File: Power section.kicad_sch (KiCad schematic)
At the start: 14 parts, among them IC1 TPD4E001RDBVR, IC2 BQ24040DSQR, J1 USB4110-GF-A, J2 B03B-PASK-1(LF)(SN)

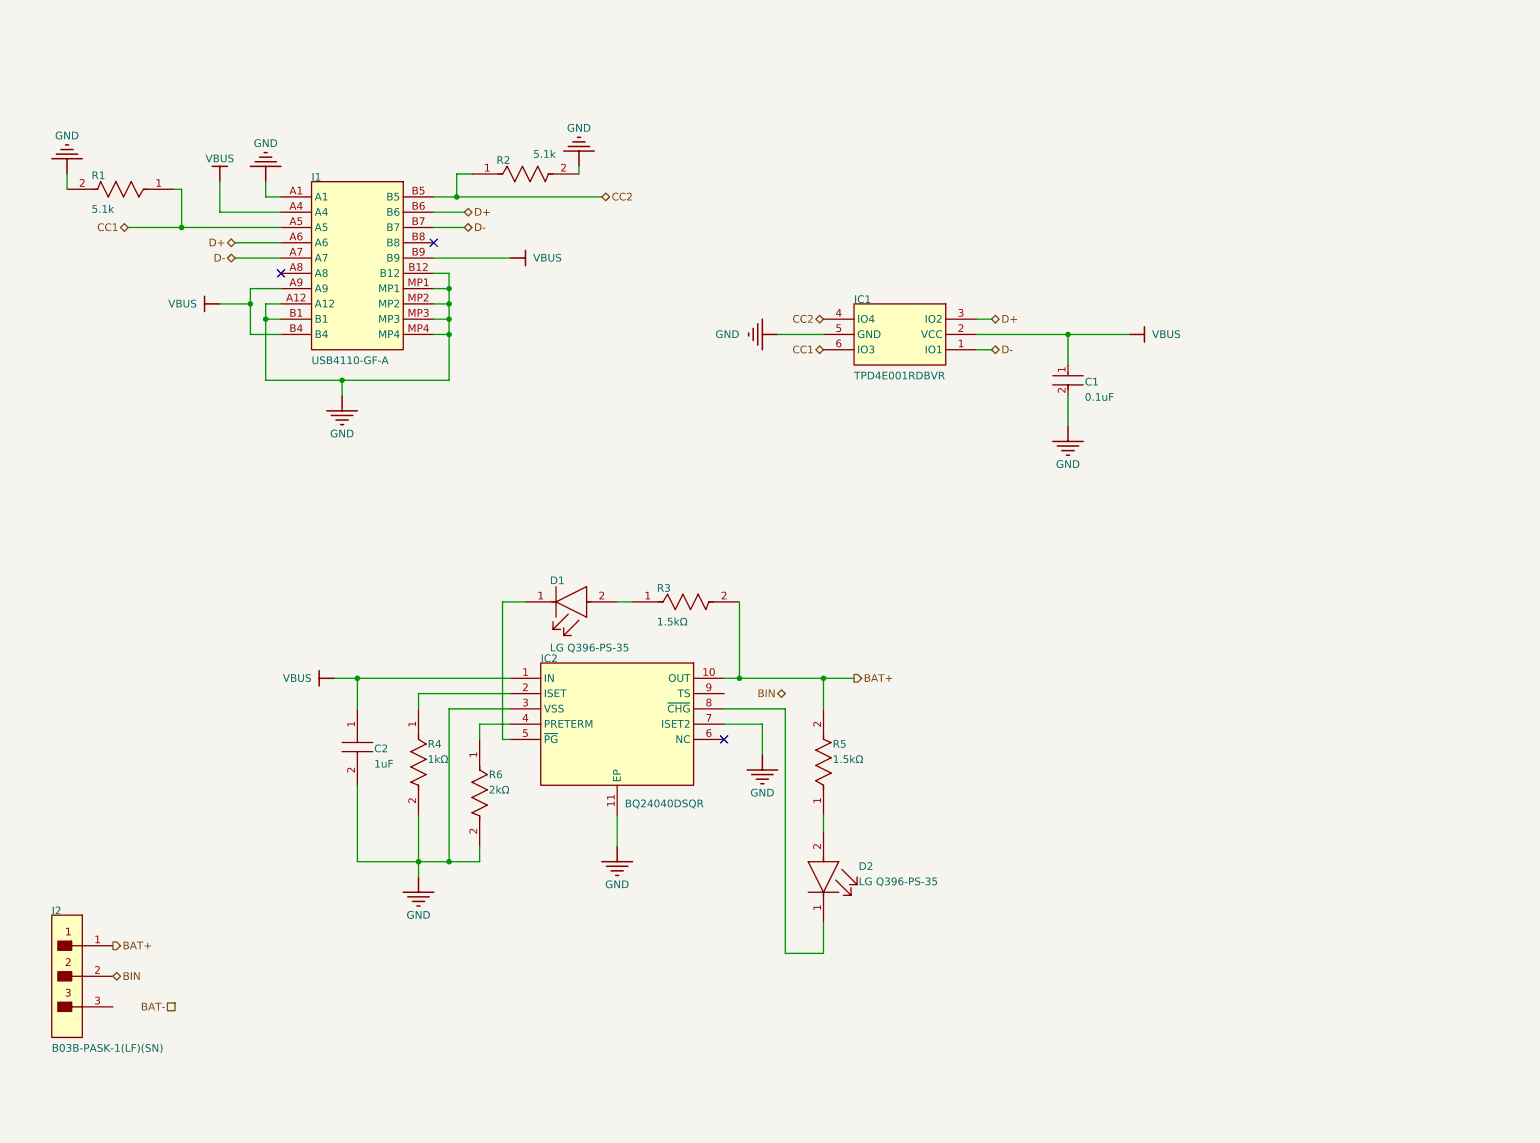
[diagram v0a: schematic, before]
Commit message: feat: schematic v1
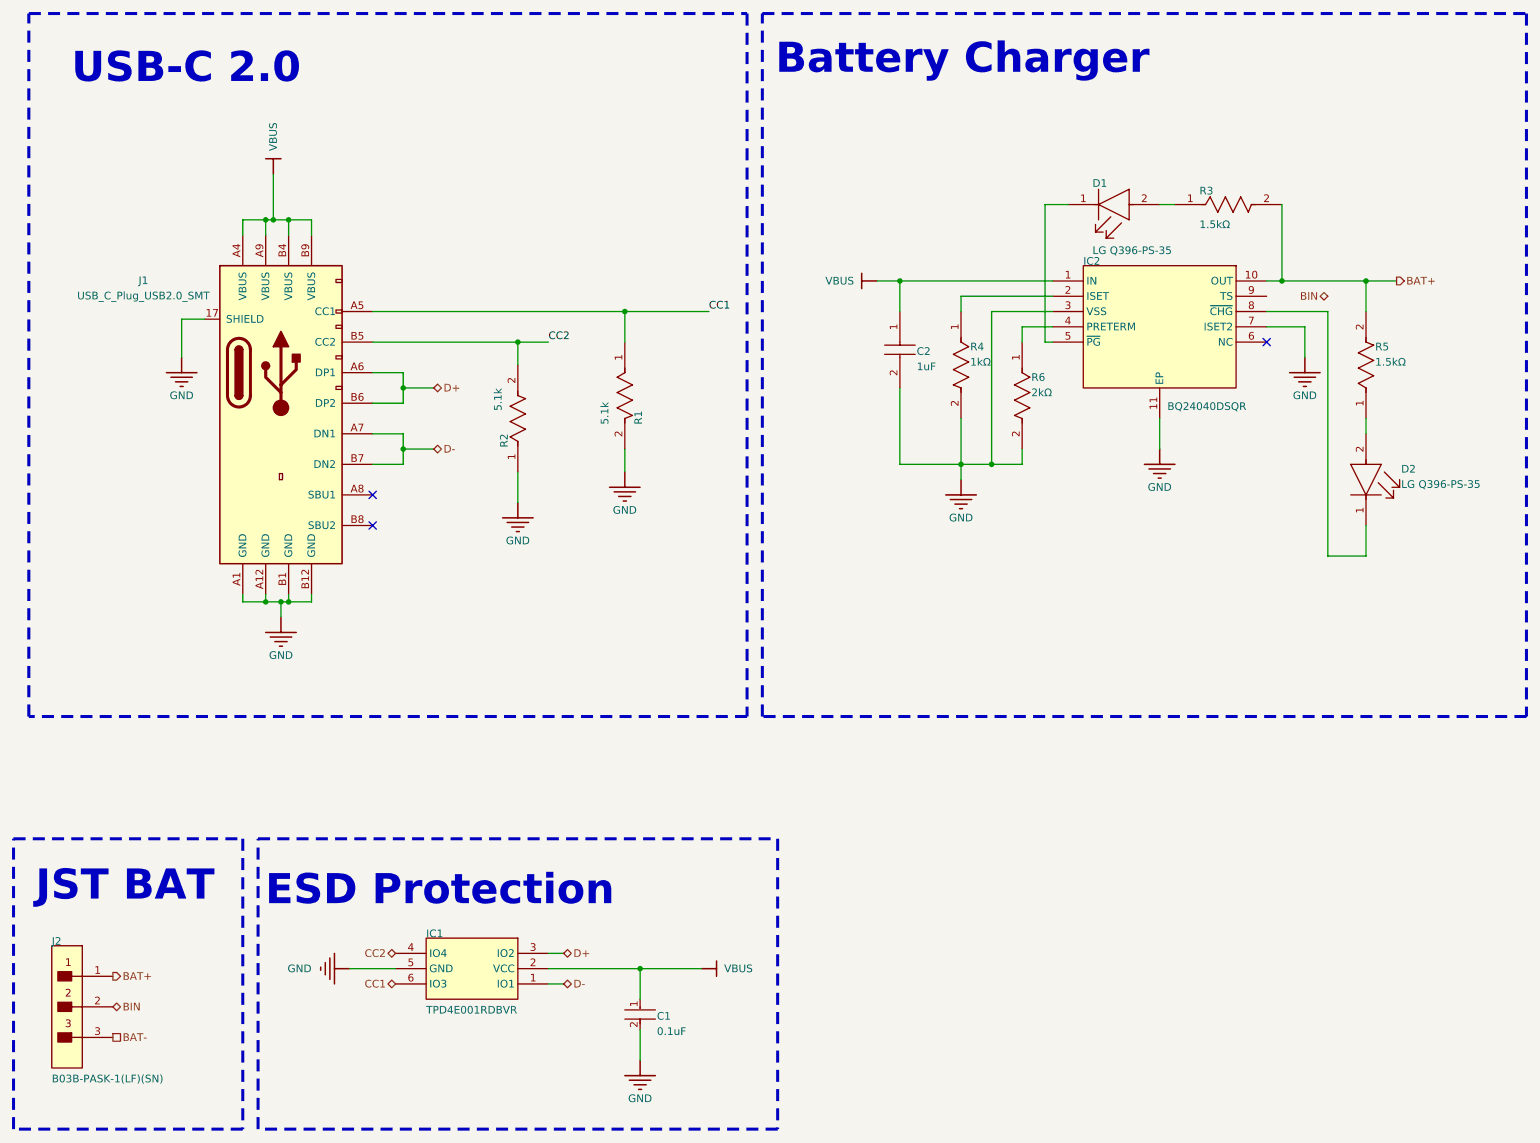
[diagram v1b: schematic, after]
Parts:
- removed J1: USB4110-GF-A, C__Users_szymo_Documents_AltiumLL_SamacSys.PcbLib:USB4110GFA, symbol *:root_0_USB4110-GF-A_*
- added J1: USB_C_Plug_USB2.0_SMT, RolandsFootprint:USB4110GFA, symbol Connectors:USB_C_Plug_USB2.0_SMT
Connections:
- net BAT-: now also J2.3
- net CC1: now also J1.A5 (CC1)
- net CC2: now also R2.2, J1.B5 (CC2); no longer R2.1
- net D+: now also J1.A6 (DP1), J1.B6 (DP2)
- net D-: now also J1.A7 (DN1), J1.B7 (DN2)
- net GND: now also R2.1, J1.17 (SHIELD), J1.A1 (GND), J1.A12 (GND), J1.B1 (GND), J1.B12 (GND); no longer R2.2
- net VBUS: now also J1.A4 (VBUS), J1.A9 (VBUS), J1.B4 (VBUS), J1.B9 (VBUS)
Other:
- note added: "Battery Charger"
- note added: "ESD Protection"
- note added: "JST BAT"
- note added: "USB-C 2.0"
- moved on the sheet: C1, C2, D1, D2, IC1, IC2, J2, R1, R2, R3, R4, R5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
